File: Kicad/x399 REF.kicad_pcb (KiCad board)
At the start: 2 copper layers, 106 x 56 mm, 84 parts, among them J1 +15V, J2 Guard, J3 10Vref, Q1 MMBT3904, Q2 2SD882, Q3 AON7410, U1 LM399, U2 OP07

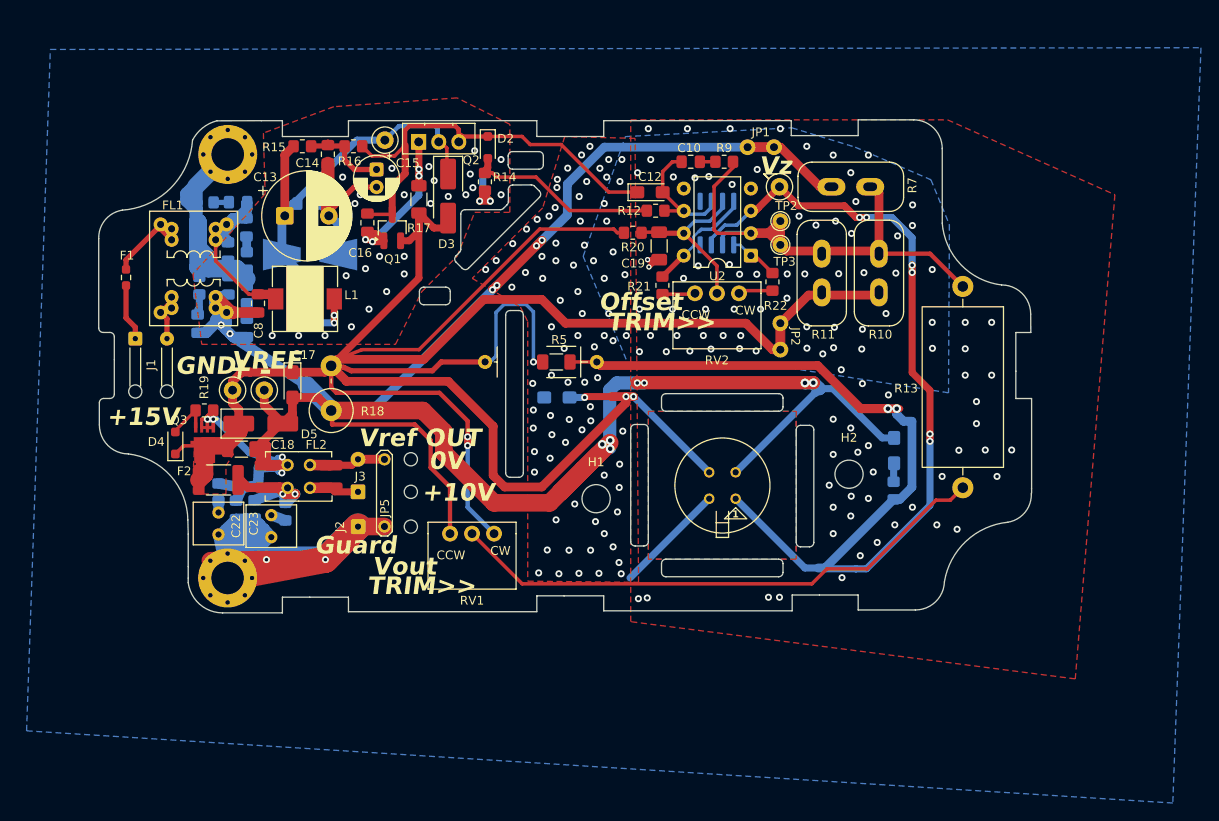
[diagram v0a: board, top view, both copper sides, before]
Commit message: Add files via upload
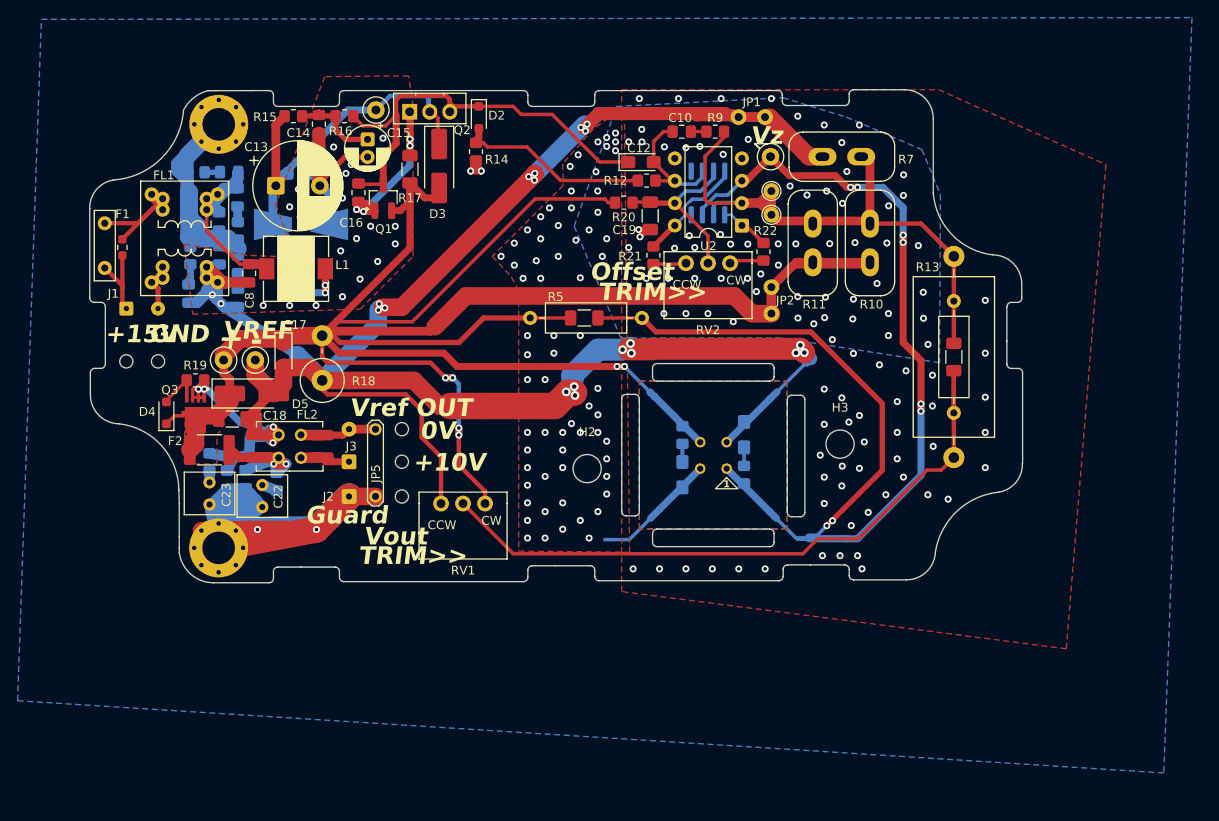
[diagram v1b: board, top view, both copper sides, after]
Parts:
- added F1alt1: RXEF010, OwnStuff:RXEF010, F.Cu at (71.0, 78.8)
- added R13alt1: 0.6W tht, Resistor_THT:R_Axial_DIN0309_L9.0mm_D3.2mm_P12.70mm_Horizontal, F.Cu at (167.4, 85.1)
- added R13alt2: 1206 smd, Resistor_SMD:R_1206_3216Metric_Pad1.30x1.75mm_HandSolder, F.Cu at (167.4, 91.4)
- added R25: 0R, Resistor_SMD:R_0805_2012Metric_Pad1.20x1.40mm_HandSolder, B.Cu at (136.6, 100.3)
- C18: value 100n NP0 -> 100n
- moved C9 17.1 mm to (143.6, 100.3)
- moved R6 17.1 mm to (143.6, 104.8)
- moved C3 16.7 mm to (136.6, 104.8), turned to -90 degrees
- moved R5 7.16 mm to (132.0, 87.0)
- moved R5alt1 5.92 mm to (125.4, 87.0)
- moved JP2 4.22 mm to (146.7, 85.0)
- moved H3 3.57 mm to (154.5, 101.3)
- moved JP1 3.57 mm to (144.5, 64.2)
- moved TP1 3.57 mm to (146.6, 68.7)
- moved C1 3.57 mm to (84.0, 76.0)
- moved C11 3.57 mm to (92.9, 70.6)
- moved C13 3.57 mm to (90.4, 72.0)
- moved C14 3.57 mm to (95.3, 65.0)
- moved C18 3.57 mm to (85.5, 98.5)
- moved C22 3.57 mm to (88.9, 108.5)
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- renumbered H3 to H1, H1 to H2, H2 to H3, R1alt1 to R5alt1
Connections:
- C3 pad 1: +10VREF -> Net-(C3-Pad1)
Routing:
- net MGND: track 343.1 -> 256.7 mm, vias 15 -> 22
- net +10VREF: track 300.7 -> 281.1 mm
- net Net-(R13-Pad2): track 62.6 -> 77.3 mm
- net Net-(JP2-A): track 12.5 -> 24.6 mm
- net Net-(U2A--): track 61.3 -> 71.2 mm
- net Net-(JP1-B): track 8.09 -> 16.0 mm
- net Net-(U2A-+): track 161.4 -> 154.6 mm
- net Net-(F1-Pad2): track 9.99 -> 15.0 mm
- net Net-(C3-Pad1): track 0.00 -> 4.12 mm
- net Net-(J1-Pin_1): track 6.47 -> 9.31 mm
- net Earth: track 83.8 -> 84.5 mm, vias 212 -> 200
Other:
- outline, holes or cut-outs redrawn
- board text added: "21-VII-2025"
- board text added: "REV {dblquote}A{dblquote}"
- board text removed: "10-VII-2025"
